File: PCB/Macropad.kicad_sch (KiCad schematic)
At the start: 29 parts, among them J1 OLED, SW1 SW_Push, SW11 RotaryEncoder_Switch, SW2 SW_Push, SW3 SW_Push, SW4 SW_Push, SW5 SW_Push, SW6 SW_Push, SW7 SW_Push, SW8 SW_Push, SW9 SW_Push, U1 XIAO-RP2040-DIP

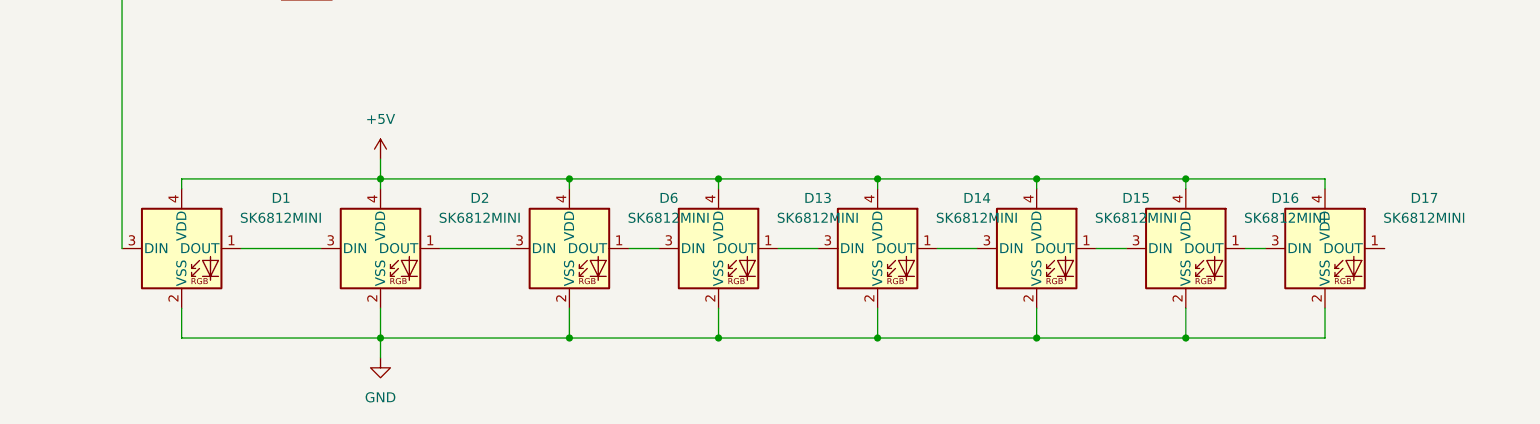
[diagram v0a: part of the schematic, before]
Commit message: Update PCB files
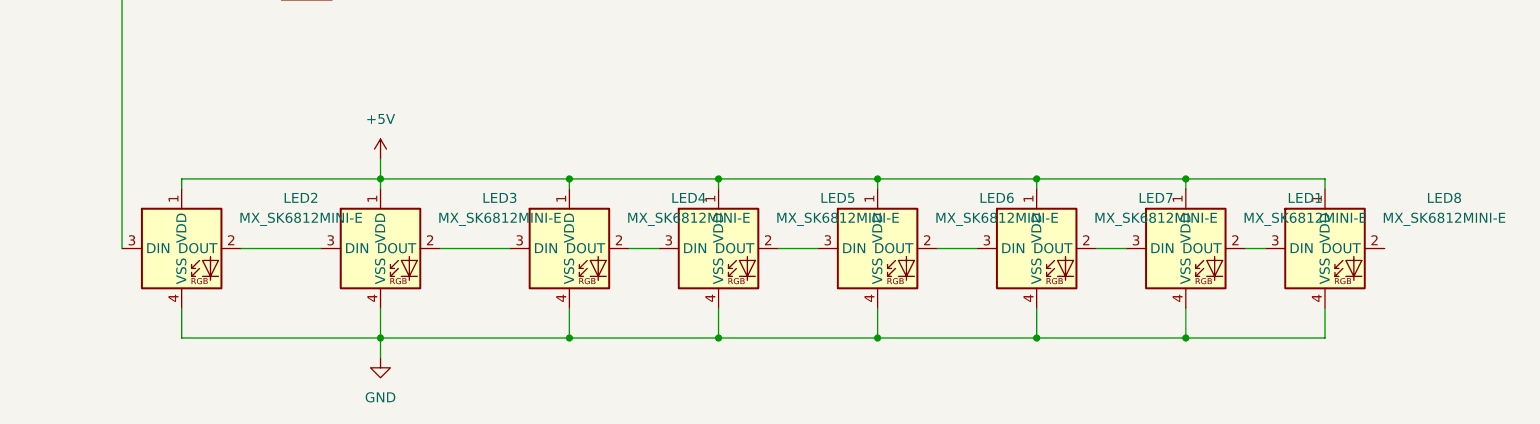
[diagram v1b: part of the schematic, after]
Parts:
- removed D1, D13, D14, D15, D16, D17, D2, D6: SK6812MINI, LED_SMD:LED_SK6812MINI_PLCC4_3.5x3.5mm_P1.75mm, symbol LED:SK6812MINI
- added LED1, LED2, LED3, LED4, LED5, LED6, LED7, LED8: MX_SK6812MINI-E, PCM_marbastlib-choc:LED_choc_6028R, symbol PCM_marbastlib-mx:MX_SK6812MINI-E
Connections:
- net +5V: now also LED1.1 (VDD), LED2.1 (VDD), LED3.1 (VDD), LED4.1 (VDD), LED5.1 (VDD), LED6.1 (VDD), LED7.1 (VDD), LED8.1 (VDD)
- net GND: now also LED1.4 (VSS), LED2.4 (VSS), LED3.4 (VSS), LED4.4 (VSS), LED5.4 (VSS), LED6.4 (VSS), LED7.4 (VSS), LED8.4 (VSS)
- net at U1.8 (GPIO1/RX): now also LED2.3 (DIN)
- new net: LED1.3 (DIN), LED7.2 (DOUT)
- new net: LED6.2 (DOUT), LED7.3 (DIN)
- new net: LED1.2 (DOUT), LED8.3 (DIN)
- new net: LED4.2 (DOUT), LED5.3 (DIN)
- new net: LED3.2 (DOUT), LED4.3 (DIN)
- new net: LED5.2 (DOUT), LED6.3 (DIN)
- new net: LED2.2 (DOUT), LED3.3 (DIN)
